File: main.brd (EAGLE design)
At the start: 36.8 x 28.6 mm, 22 parts, among them Y1 16MHz

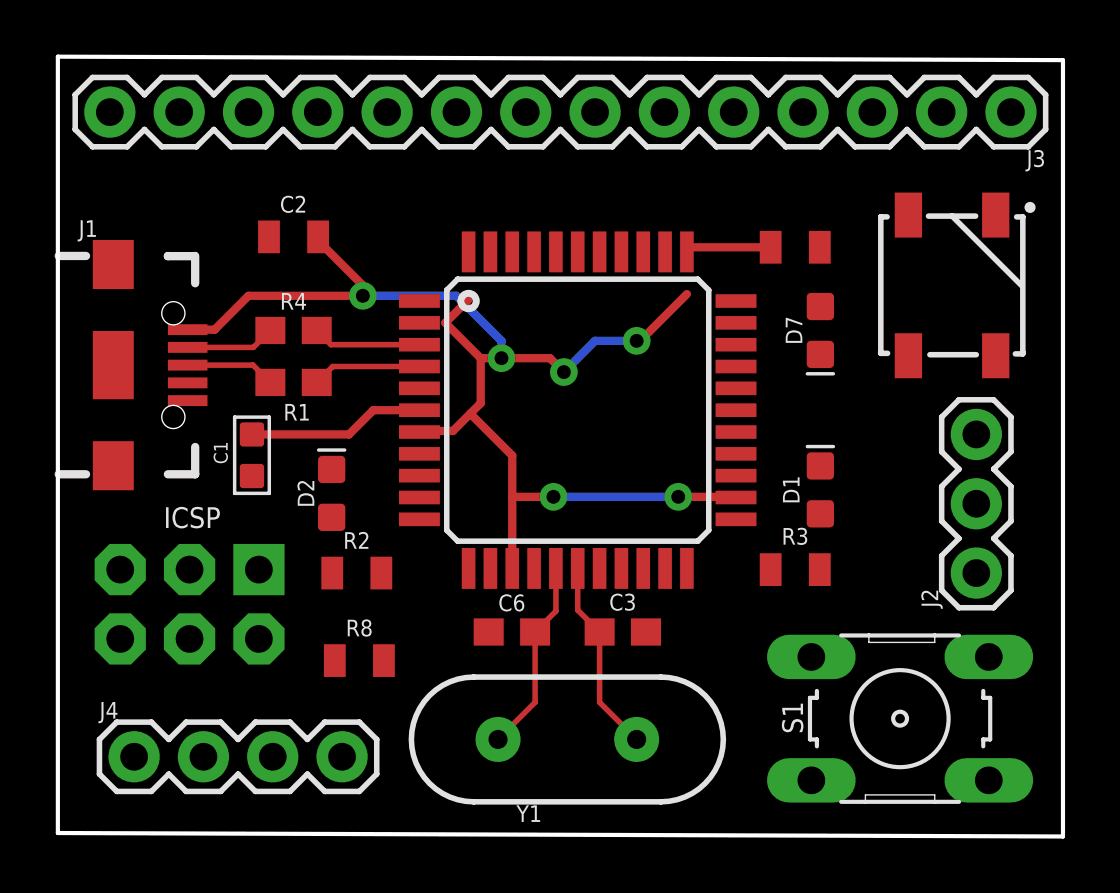
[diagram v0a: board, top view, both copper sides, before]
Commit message: Move vias
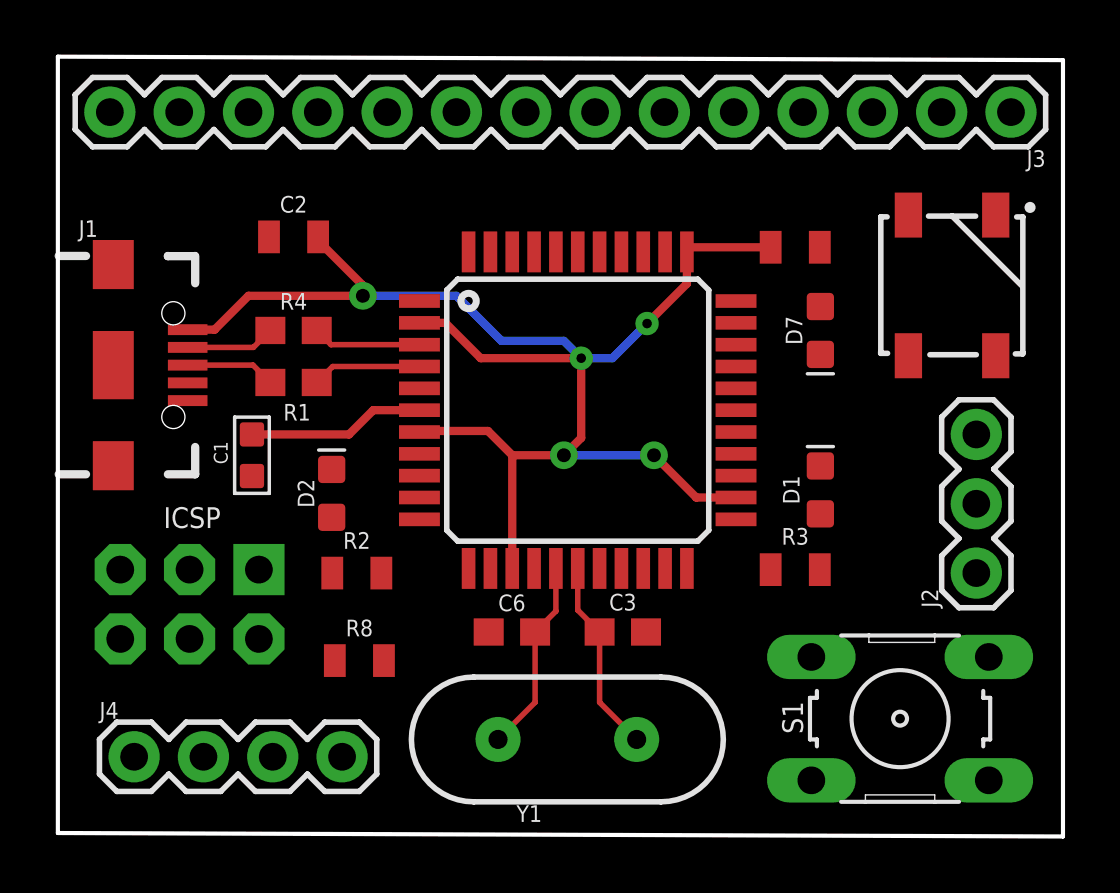
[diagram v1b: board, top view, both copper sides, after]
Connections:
- net RX_N renamed TX
- net RX_P renamed RX
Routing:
- net 5V: track 49.7 -> 54.7 mm, vias 6 -> 5
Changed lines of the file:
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@@
 <via x="11.176" y="23.241" extent="1-16" drill="0.508"/>
 <wire x1="11.176" y1="23.241" x2="14.605" y2="23.241" width="0.3048" layer="16"/>
-<wire x1="14.605" y1="23.241" x2="16.256" y2="21.59" width="0.3048" layer="16"/>
-<wire x1="16.256" y1="21.59" x2="16.256" y2="20.955" width="0.3048" layer="16"/>
-<via x="16.256" y="20.955" extent="1-16" drill="0.508"/>
+<wire x1="16.256" y1="21.59" x2="14.605" y2="23.241" width="0.3048" layer="16"/>
 <wire x1="14.199" y1="22.25" x2="15.494" y2="20.955" width="0.3048" layer="1"/>
-<wire x1="15.494" y1="20.955" x2="16.256" y2="20.955" width="0.3048" layer="1"/>
-<wire x1="15.494" y1="20.955" x2="15.494" y2="19.304" width="0.3048" layer="1"/>
-<wire x1="15.494" y1="19.304" x2="14.478" y2="18.288" width="0.3048" layer="1"/>
-<wire x1="14.478" y1="18.288" x2="13.288" y2="18.288" width="0.3048" layer="1"/>
-<wire x1="15.05" y1="23.101" x2="14.199" y2="22.25" width="0.3048" layer="1"/>
-<wire x1="23.05" y1="23.304" x2="21.336" y2="21.59" width="0.3048" layer="1"/>
-<wire x1="21.336" y1="21.59" x2="21.209" y2="21.59" width="0.3048" layer="1"/>
-<via x="21.209" y="21.59" extent="1-16" drill="0.508"/>
-<wire x1="21.209" y1="21.59" x2="19.685" y2="21.59" width="0.3048" layer="16"/>
-<wire x1="19.685" y1="21.59" x2="18.542" y2="20.447" width="0.3048" layer="16"/>
-<via x="18.542" y="20.447" extent="1-16" drill="0.508"/>
-<wire x1="16.256" y1="20.955" x2="18.034" y2="20.955" width="0.3048" layer="1"/>
-<wire x1="18.034" y1="20.955" x2="18.542" y2="20.447" width="0.3048" layer="1"/>
 <wire x1="11.176" y1="23.622" x2="11.176" y2="23.241" width="0.3048" layer="1"/>
 <wire x1="9.536" y1="25.262" x2="11.176" y2="23.622" width="0.3048" layer="1"/>
@@
 <contactref element="U$1" pad="24"/>
 <contactref element="U$1" pad="44"/>
-<wire x1="15.113" y1="18.923" x2="16.65" y2="17.386" width="0.3048" layer="1"/>
-<wire x1="16.65" y1="15.87493125" x2="16.65" y2="13.25" width="0.3048" layer="1"/>
-<wire x1="16.65" y1="15.87493125" x2="16.65" y2="17.386" width="0.3048" layer="1"/>
-<wire x1="24.825" y1="15.875" x2="24.85" y2="15.85" width="0.3048" layer="1"/>
-<wire x1="24.825" y1="15.875" x2="22.733" y2="15.875" width="0.3048" layer="1"/>
-<via x="22.733" y="15.875" extent="1-16" drill="0.508"/>
-<wire x1="22.733" y1="15.875" x2="18.161" y2="15.875" width="0.3048" layer="16"/>
-<via x="18.161" y="15.875" extent="1-16" drill="0.508"/>
-<wire x1="18.161" y1="15.875" x2="18.16093125" y2="15.87493125" width="0.3048" layer="1"/>
-<wire x1="18.16093125" y1="15.87493125" x2="16.65" y2="15.87493125" width="0.3048" layer="1"/>
+<wire x1="16.65" y1="17.39893125" x2="16.65" y2="13.25" width="0.3048" layer="1"/>
+<wire x1="24.85" y1="15.85" x2="24.825" y2="15.875" width="0.3048" layer="1"/>
+<via x="21.844" y="17.399" extent="1-16" drill="0.508"/>
+<via x="18.542" y="17.399" extent="1-16" drill="0.508"/>
 <contactref element="U$1" pad="7"/>
 <contactref element="U$1" pad="2"/>
 <contactref element="C2" pad="2"/>
 <contactref element="J3" pad="14"/>
+<wire x1="18.542" y1="17.399" x2="18.54193125" y2="17.39893125" width="0.3048" layer="1"/>
+<wire x1="16.65" y1="17.39893125" x2="18.54193125" y2="17.39893125" width="0.3048" layer="1"/>
+<wire x1="18.542" y1="17.399" x2="21.844" y2="17.399" width="0.3048" layer="16"/>
+<wire x1="21.844" y1="17.399" x2="23.393" y2="15.85" width="0.3048" layer="1"/>
+<wire x1="23.393" y1="15.85" x2="24.85" y2="15.85" width="0.3048" layer="1"/>
+<wire x1="14.199" y1="22.25" x2="13.25" y2="22.25" width="0.3048" layer="1"/>
+<wire x1="15.494" y1="20.955" x2="19.177" y2="20.955" width="0.3048" layer="1"/>
+<via x="19.177" y="20.955" extent="1-16" drill="0.35"/>
+<wire x1="18.542" y1="21.59" x2="19.177" y2="20.955" width="0.3048" layer="16"/>
+<wire x1="18.542" y1="21.59" x2="16.256" y2="21.59" width="0.3048" layer="16"/>
+<wire x1="15.76093125" y1="18.288" x2="16.65" y2="17.39893125" width="0.3048" layer="1"/>
+<wire x1="13.288" y1="18.288" x2="15.76093125" y2="18.288" width="0.3048" layer="1"/>
+<wire x1="19.177" y1="20.955" x2="19.177" y2="18.034" width="0.3048" layer="1"/>
+<wire x1="19.177" y1="18.034" x2="18.542" y2="17.399" width="0.3048" layer="1"/>
+<wire x1="19.177" y1="20.955" x2="20.32" y2="20.955" width="0.3048" layer="16"/>
+<wire x1="20.32" y1="20.955" x2="21.59" y2="22.225" width="0.3048" layer="16"/>
+<via x="21.59" y="22.225" extent="1-16" drill="0.35"/>
+<wire x1="21.59" y1="22.225" x2="23.05" y2="23.685" width="0.3048" layer="1"/>
+<wire x1="23.05" y1="23.685" x2="23.05" y2="24.85" width="0.3048" layer="1"/>
 <wire x1="26.11925" y1="25.019" x2="31.166" y2="21.045" width="0" layer="19" extent="1-1"/>
 <wire x1="23.05" y1="24.85" x2="23.219" y2="25.019" width="0" layer="19" extent="1-1"/>
-<wire x1="23.05" y1="23.304" x2="23.05" y2="24.85" width="0" layer="19" extent="1-1"/>
 <wire x1="13.25" y1="18.25" x2="13.288" y2="18.288" width="0" layer="19" extent="1-1"/>
 <wire x1="9.536" y1="25.4" x2="9.536" y2="25.262" width="0" layer="19" extent="1-1"/>
-<wire x1="15.113" y1="18.923" x2="15.494" y2="19.304" width="0" layer="19" extent="1-1"/>
-<wire x1="13.25" y1="22.25" x2="14.199" y2="22.25" width="0" layer="19" extent="1-1"/>
 <wire x1="15.05" y1="24.85" x2="14.605" y2="23.241" width="0" layer="19" extent="1-16"/>
 <wire x1="11.949" y1="9.87425" x2="16.65" y2="13.25" width="0" layer="19" extent="1-1"/>
@@
 <wire x1="13.25" y1="21.45" x2="10.007" y2="21.45" width="0.2032" layer="1"/>
 <wire x1="10.007" y1="21.45" x2="9.486" y2="21.971" width="0.2032" layer="1"/>
-</signal>
-<signal name="RX_P">
-<contactref element="U$1" pad="20"/>
-<contactref element="J4" pad="3"/>
-<wire x1="7.874" y1="6.35" x2="21.45" y2="13.25" width="0" layer="19" extent="1-1"/>
-</signal>
-<signal name="RX_N">
-<contactref element="U$1" pad="21"/>
-<contactref element="J4" pad="4"/>
-<wire x1="10.414" y1="6.35" x2="22.25" y2="13.25" width="0" layer="19" extent="1-1"/>
 </signal>
 <signal name="PC7">
@@
 <wire x1="24.85" y1="21.45" x2="27.305" y2="29.972" width="0" layer="19" extent="1-1"/>
 </signal>
+<signal name="RX">
+<contactref element="U$1" pad="20"/>
+<contactref element="J4" pad="3"/>
+<wire x1="7.874" y1="6.35" x2="21.45" y2="13.25" width="0" layer="19" extent="1-1"/>
+</signal>
+<signal name="TX">
+<contactref element="U$1" pad="21"/>
+<contactref element="J4" pad="4"/>
+<wire x1="10.414" y1="6.35" x2="22.25" y2="13.25" width="0" layer="19" extent="1-1"/>
+</signal>
 </signals>
